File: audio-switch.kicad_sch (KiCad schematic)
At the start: 26 parts, among them U7 FST3257

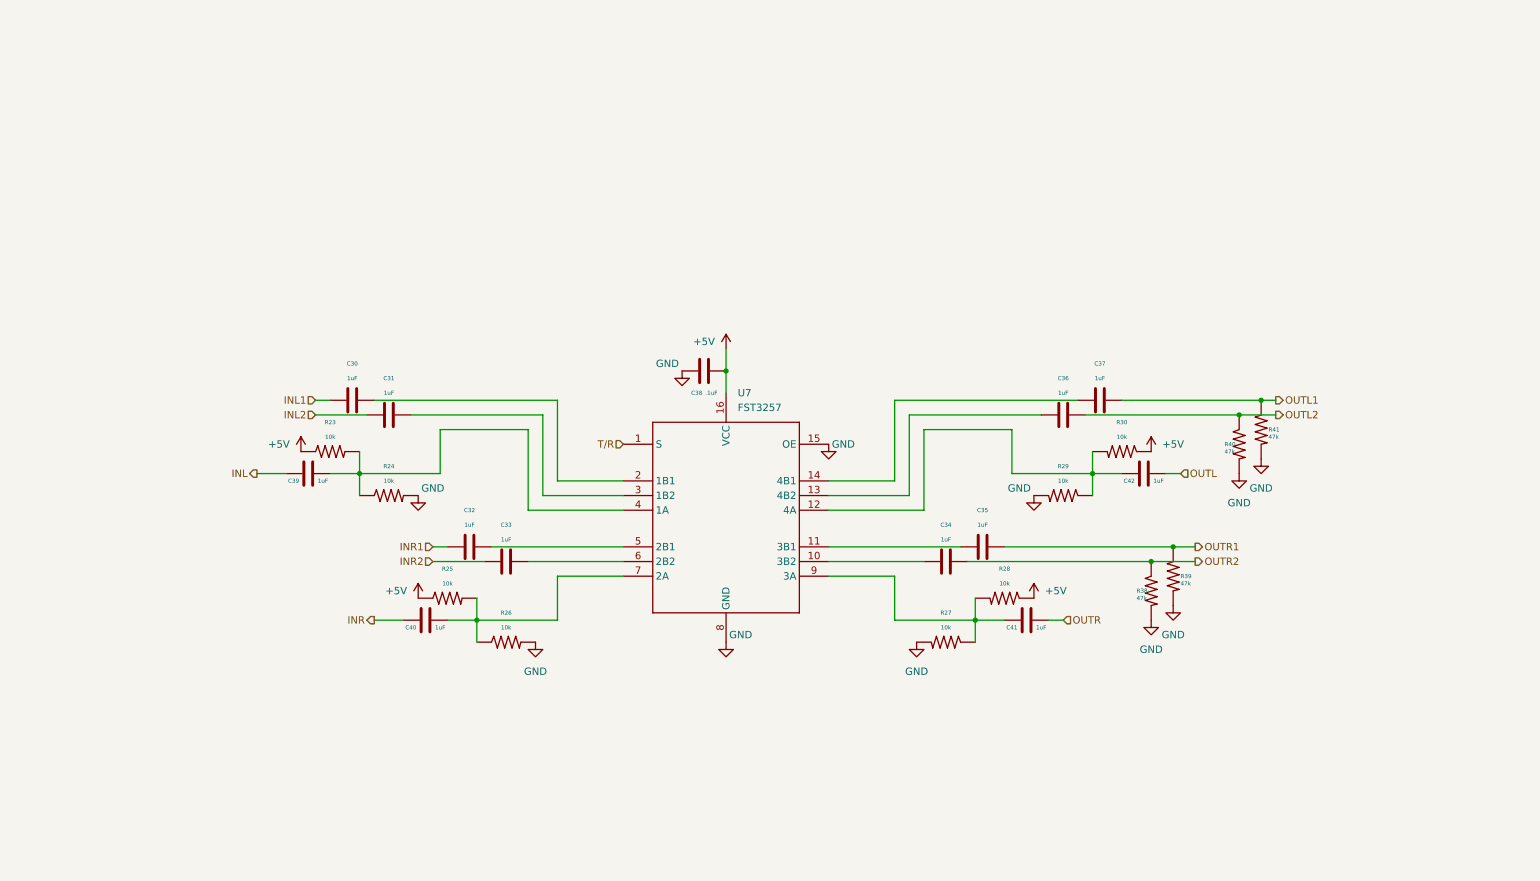
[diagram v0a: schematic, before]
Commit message: Add files via upload
Added "WIP" branch, which is some of my mods.
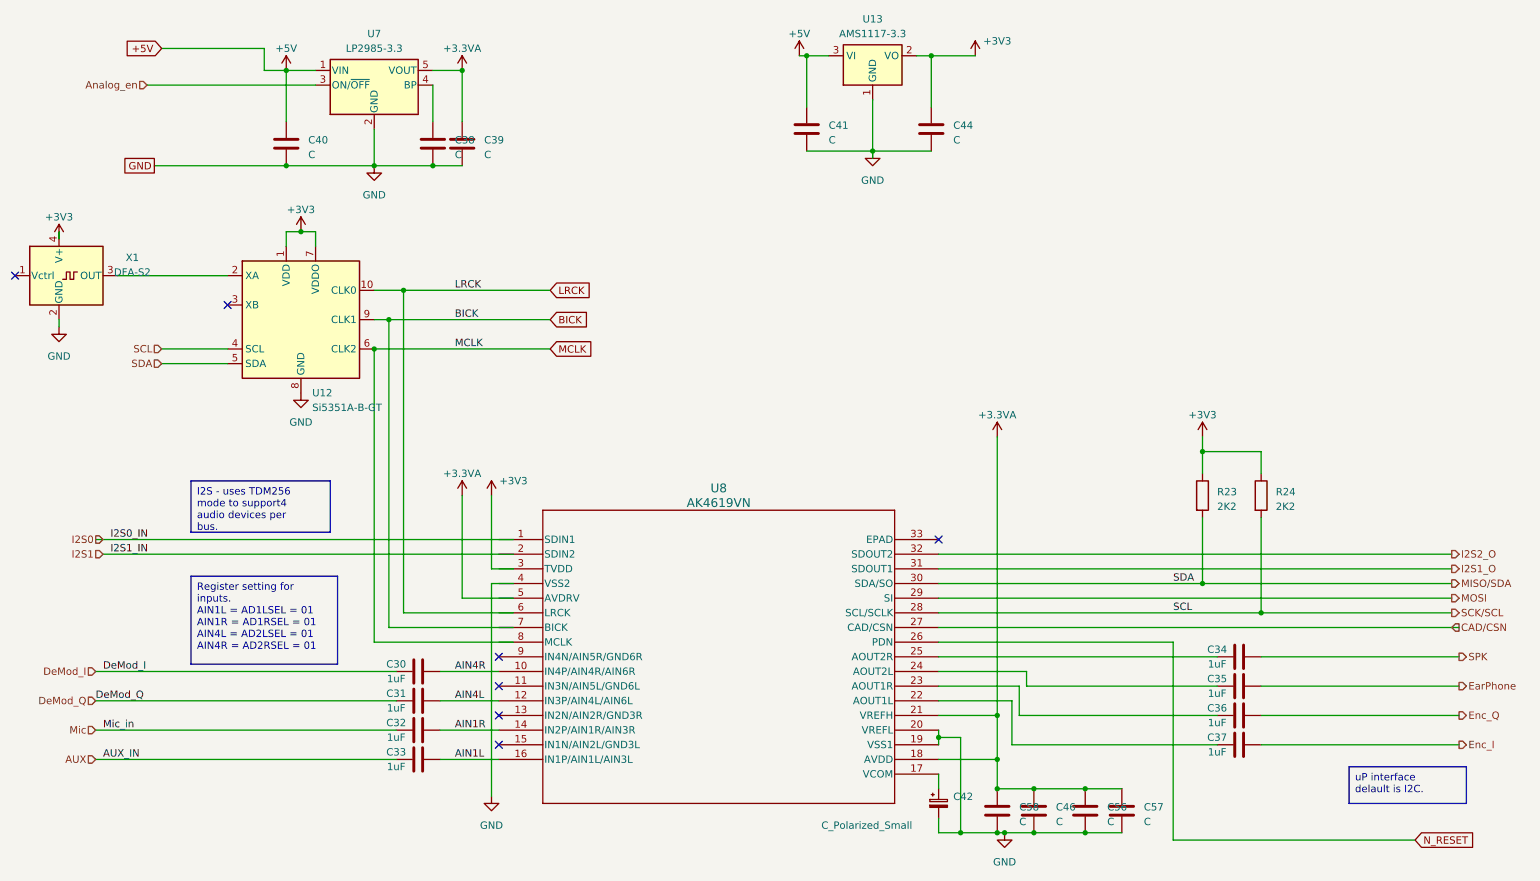
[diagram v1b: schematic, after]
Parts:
- removed C30, C31, C32, C33, C34, C35, C36, C37, C39, C40, C41, C42: 1uF, Capacitor_SMD:C_0805_2012Metric, symbol Xenir:Capacitor
- removed C38: .1uF, Capacitor_SMD:C_0805_2012Metric, symbol Xenir:Capacitor
- removed R23, R24, R25, R26, R27, R28, R29, R30: 10k, Resistor_SMD:R_0805_2012Metric, symbol Xenir:Resistor
- removed R38, R39, R40, R41: 47k, Resistor_SMD:R_0805_2012Metric, symbol Xenir:Resistor
- removed U7: FST3257, Xenir:SO16, symbol Xenir_v6:FST3257
- added C30, C31, C32, C33, C34, C35, C36, C37: 1uF, symbol Device:C
- added C38, C39, C40, C41, C44, C46, C56, C57, C58: C, symbol Device:C
- added C42: C_Polarized_Small, symbol Device:C_Polarized_Small
- added R23, R24: 2K2, Resistor_SMD:R_0805_2012Metric_Pad1.20x1.40mm_HandSolder, symbol Device:R
- added U12: Si5351A-B-GT, Package_SO:MSOP-10_3x3mm_P0.5mm, symbol Oscillator:Si5351A-B-GT
- added U13: AMS1117-3.3, Package_TO_SOT_SMD:SOT-223-3_TabPin2, symbol Regulator_Linear:AMS1117-3.3
- added U7: LP2985-3.3, Package_TO_SOT_SMD:SOT-23-5, symbol Regulator_Linear:LP2985-3.3
- added U8: AK4619VN, AK4619VN_AKM, symbol AK4619VN:AK4619VN
- added X1: DFA-S2, Oscillator:Oscillator_SMD_Fordahl_DFAS2-4Pin_7.3x5.1mm, symbol Oscillator:DFA-S2
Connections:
- net +5V: now also C40.2, C41.2, U13.3 (VI), U7.1 (VIN)
- net GND: now also C38.1, C39.1, C40.1, C41.1, C42.2, C44.1, C46.2, C56.2, C57.2, C58.2, U12.8 (GND), U13.1 (GND), U7.2 (GND), U8.19 (VSS1), U8.20 (VREFL), X1.2 (GND)
- new net: C35.1, U8.24 (AOUT2L)
- new net: C37.1, U8.22 (AOUT1L)
- new net: C34.1, U8.25 (AOUT2R)
- new net: U12.2 (XA), X1.3 (OUT)
- new net: C42.1, U8.17 (VCOM)
- new net: C38.2, U7.4 (BP)
- new net: C36.1, U8.23 (AOUT1R)
- new net +3.3VA: C39.2, C46.1, C56.1, C57.1, C58.1, U7.5 (VOUT), U8.18 (AVDD), U8.21 (VREFH)
- new net +3V3: C44.2, R23.1, R24.1, U12.1 (VDD), U12.7 (VDDO), U13.2 (VO), X1.4 (V+)
- new net AIN1L: C33.2, U8.16 (IN1P/AIN1L/AIN3L)
- new net AIN1R: C32.2, U8.14 (IN2P/AIN1R/AIN3R)
- new net AIN4L: C31.2, U8.12 (IN3P/AIN4L/AIN6L)
- new net AIN4R: C30.2, U8.10 (IN4P/AIN4R/AIN6R)
- new net AUX: C33.1
- new net Analog_en: U7.3 (ON/~{OFF})
- new net BICK: U12.9 (CLK1)
- new net CAD/CSN: U8.27 (CAD/CSN)
- new net DeMod_I: C30.1
- new net DeMod_Q: C31.1
- new net EarPhone: C35.2
- new net Enc_I: C37.2
- new net Enc_Q: C36.2
- new net I2S1_O: U8.31 (SDOUT1)
- new net I2S2_O: U8.32 (SDOUT2)
- new net LRCK: U12.10 (CLK0)
- new net MCLK: U12.6 (CLK2)
- new net MISO/SDA: R23.2, U12.5 (SDA), U8.30 (SDA/SO)
- new net MOSI: U8.29 (SI)
- new net Mic: C32.1
- new net N_RESET: U8.26 (PDN)
- new net SCK/SCL: R24.2, U12.4 (SCL), U8.28 (SCL/SCLK)
- new net SPK: C34.2
- no-connect marks 0 -> 7
